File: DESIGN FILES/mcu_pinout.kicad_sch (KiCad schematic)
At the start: 16 parts, among them U1 MIMXRT1064CVL5B

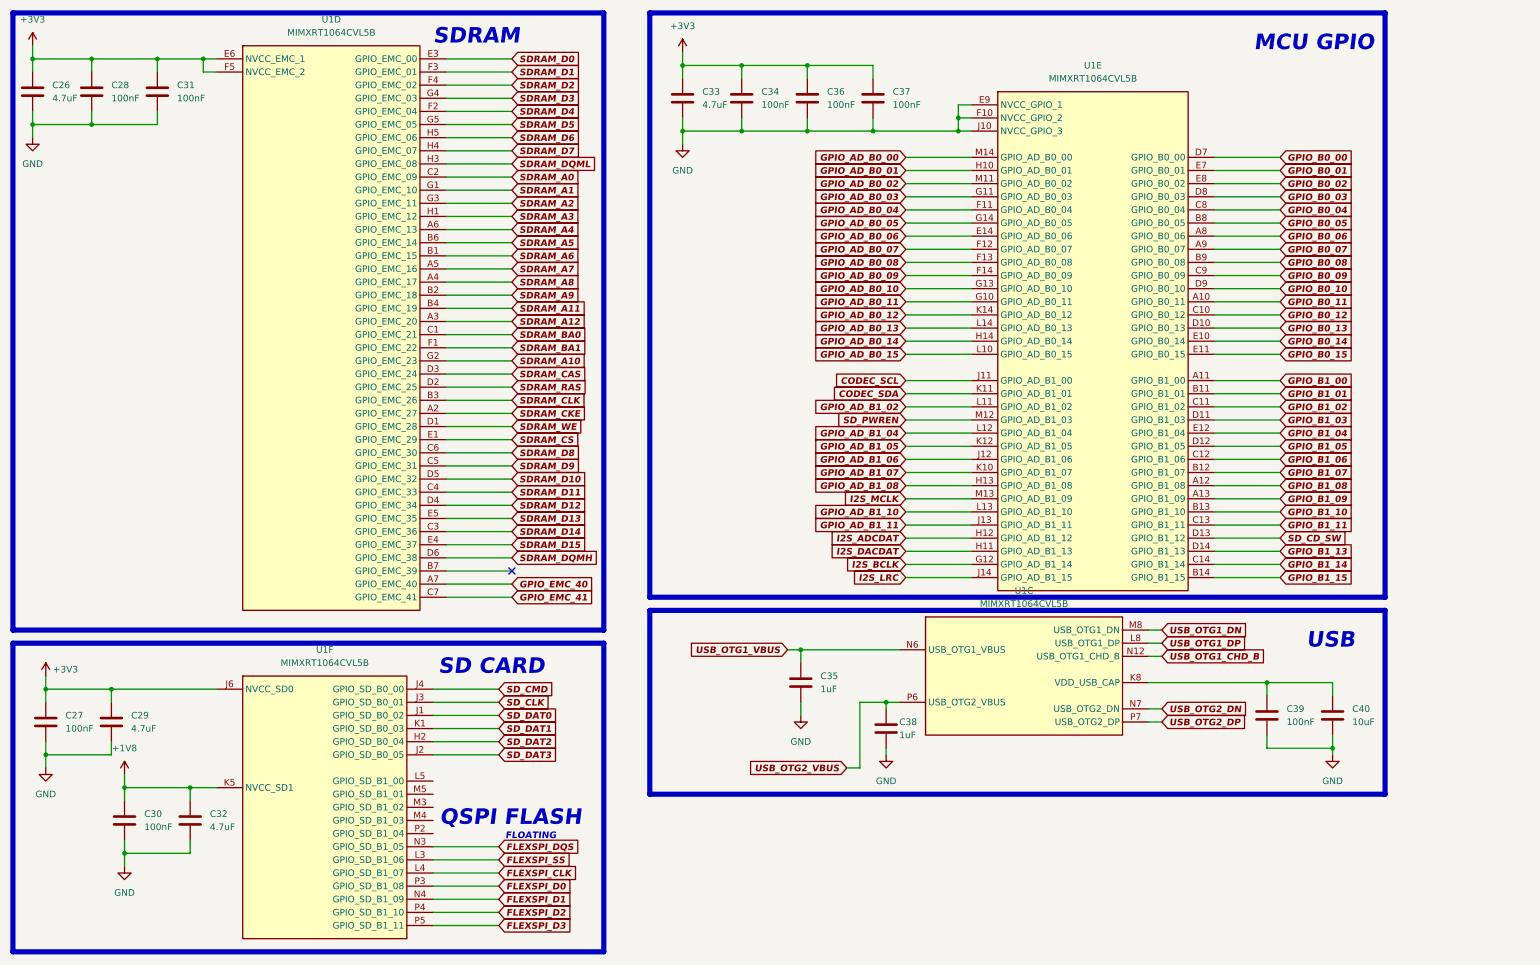
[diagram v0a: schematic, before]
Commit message: work
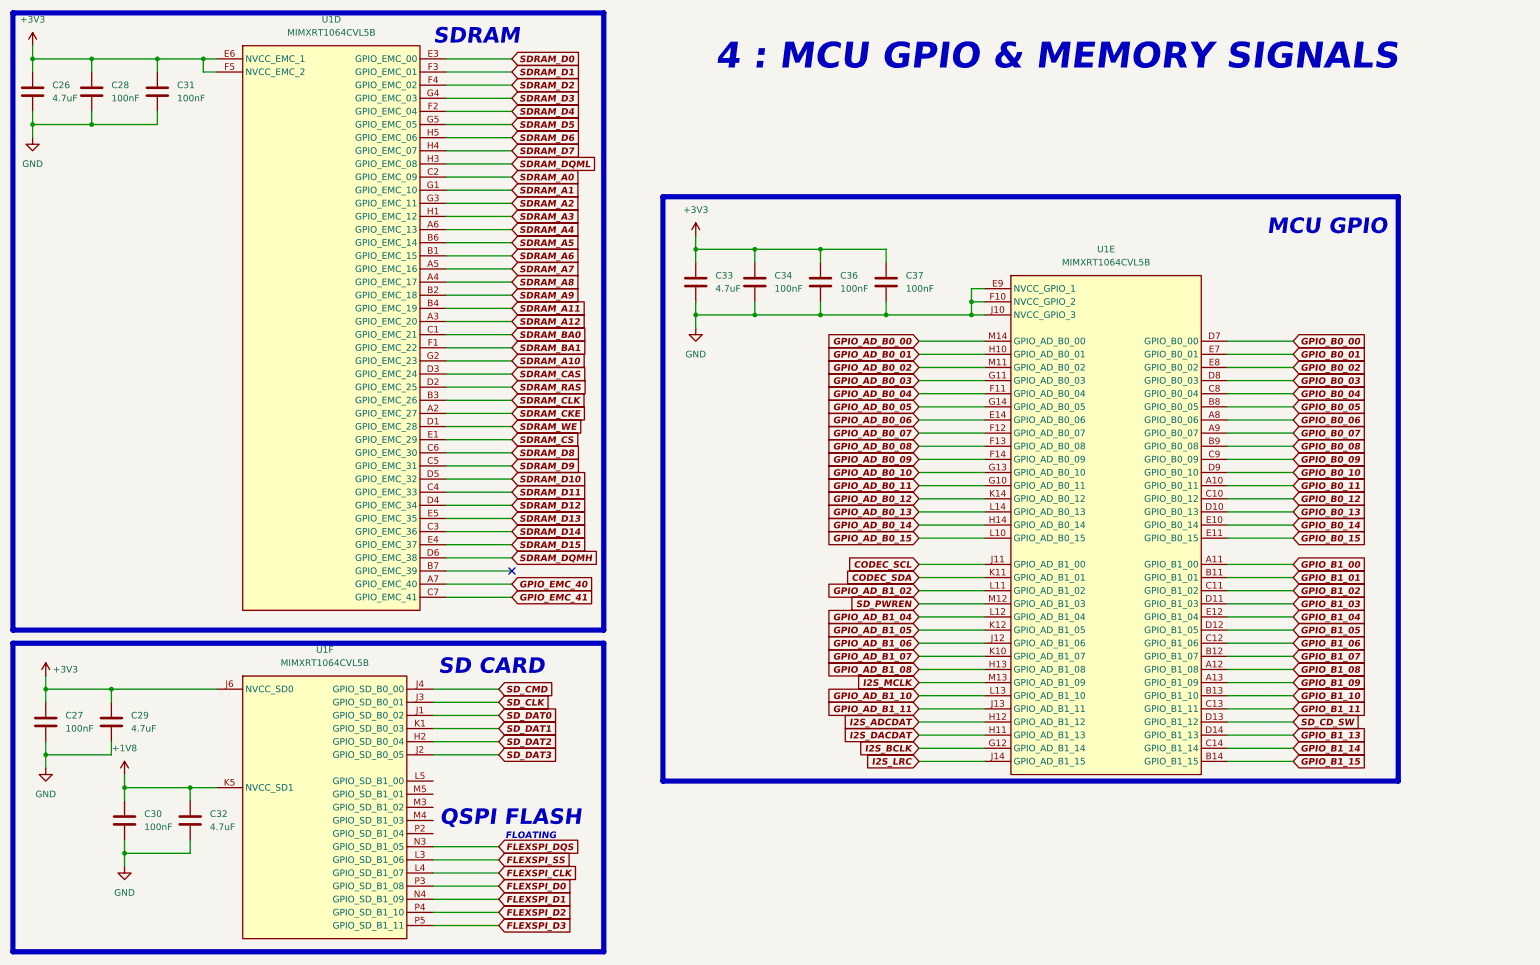
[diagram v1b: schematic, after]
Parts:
- removed C35, C38: 1uF, MIMXRT1064 MCU Module:0402_CL05A105KA5NQNC, symbol MIMXRT1064 MCU Module:CL05A105KA5NQNC
- removed C39: 100nF, MIMXRT1064 MCU Module:0402_CL05B104KB54PNC, symbol MIMXRT1064 MCU Module:CL05B104KB54PNC
- removed C40: 10uF, MIMXRT1064 MCU Module:0603_CL10A106KP8NNNC, symbol MIMXRT1064 MCU Module:CL10A106KP8NNNC
- removed unit 3 of U1
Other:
- note added: "4 : MCU GPIO & MEMORY SIGNALS"
- note removed: "USB"
- company: (none) -> Soundsom
- title: (none) -> MCU GPIO & Memory signals
- moved on the sheet: C33, C34, C36, C37, U1E

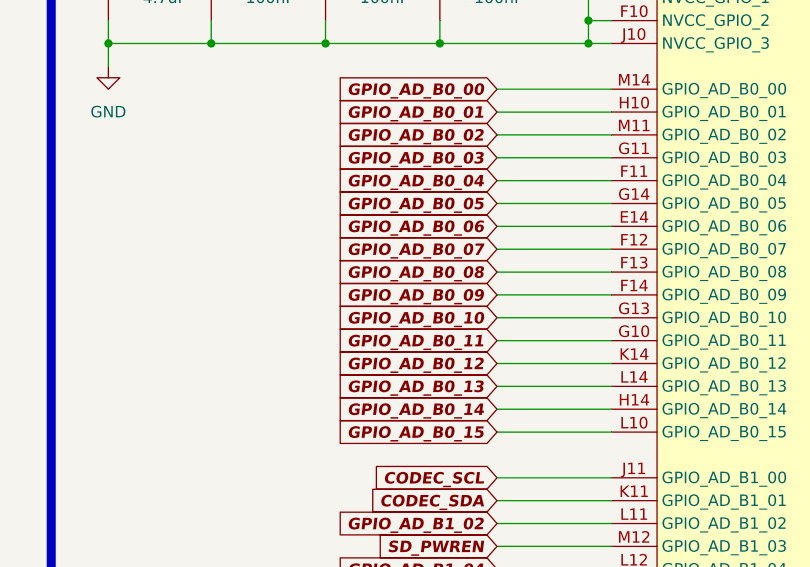
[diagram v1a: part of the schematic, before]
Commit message: schematic edit
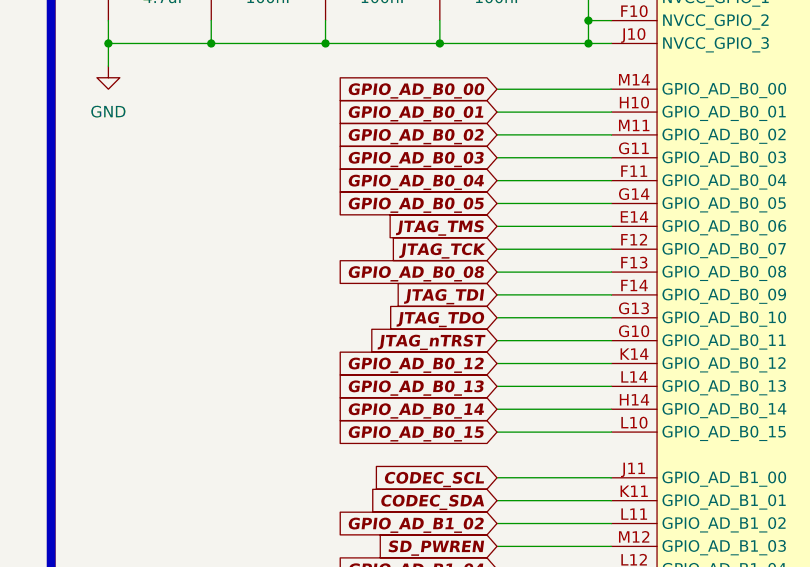
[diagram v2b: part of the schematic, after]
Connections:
- net GPIO_AD_B0_06 renamed JTAG_TMS
- net GPIO_AD_B0_07 renamed JTAG_TCK
- net GPIO_AD_B0_09 renamed JTAG_TDI
- net GPIO_AD_B0_10 renamed JTAG_TDO
- net GPIO_AD_B0_11 renamed JTAG_nTRST
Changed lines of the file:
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@@
     )
   )
-  (global_label "GPIO_AD_B0_06" (shape input) (at 189.23 92.71 180) (fields_autoplaced)
-    (effects (font (size 1.27 1.27) bold italic) (justify right))
-    (property "Intersheet References" "${INTERSHEET_REFS}" (id 0) (at 171.7357 92.583 0)
+  (global_label "JTAG_TMS" (shape input) (at 189.23 92.71 180) (fields_autoplaced)
+    (effects (font (size 1.27 1.27) bold italic) (justify right))
+    (property "Intersheet References" "${INTERSHEET_REFS}" (id 0) (at 177.4809 92.583 0)
       (effects (font (size 1.27 1.27) bold italic) (justify right) hide)
     )
@@
     )
   )
-  (global_label "GPIO_AD_B0_09" (shape input) (at 189.23 100.33 180) (fields_autoplaced)
-    (effects (font (size 1.27 1.27) bold italic) (justify right))
-    (property "Intersheet References" "${INTERSHEET_REFS}" (id 0) (at 171.7357 100.203 0)
+  (global_label "JTAG_TDI" (shape input) (at 189.23 100.33 180) (fields_autoplaced)
+    (effects (font (size 1.27 1.27) bold italic) (justify right))
+    (property "Intersheet References" "${INTERSHEET_REFS}" (id 0) (at 178.2671 100.203 0)
       (effects (font (size 1.27 1.27) bold italic) (justify right) hide)
     )
@@
     )
   )
-  (global_label "GPIO_AD_B0_10" (shape input) (at 189.23 102.87 180) (fields_autoplaced)
-    (effects (font (size 1.27 1.27) bold italic) (justify right))
-    (property "Intersheet References" "${INTERSHEET_REFS}" (id 0) (at 171.7357 102.743 0)
+  (global_label "JTAG_TDO" (shape input) (at 189.23 102.87 180) (fields_autoplaced)
+    (effects (font (size 1.27 1.27) bold italic) (justify right))
+    (property "Intersheet References" "${INTERSHEET_REFS}" (id 0) (at 177.5414 102.743 0)
       (effects (font (size 1.27 1.27) bold italic) (justify right) hide)
     )
@@
     )
   )
-  (global_label "GPIO_AD_B0_11" (shape input) (at 189.23 105.41 180) (fields_autoplaced)
-    (effects (font (size 1.27 1.27) bold italic) (justify right))
-    (property "Intersheet References" "${INTERSHEET_REFS}" (id 0) (at 171.7357 105.283 0)
+  (global_label "JTAG_nTRST" (shape input) (at 189.23 105.41 180) (fields_autoplaced)
+    (effects (font (size 1.27 1.27) bold italic) (justify right))
+    (property "Intersheet References" "${INTERSHEET_REFS}" (id 0) (at 175.5457 105.283 0)
       (effects (font (size 1.27 1.27) bold italic) (justify right) hide)
     )
@@
     )
   )
-  (global_label "GPIO_AD_B0_07" (shape input) (at 189.23 95.25 180) (fields_autoplaced)
-    (effects (font (size 1.27 1.27) bold italic) (justify right))
-    (property "Intersheet References" "${INTERSHEET_REFS}" (id 0) (at 171.7357 95.123 0)
-      (effects (font (size 1.27 1.27) bold italic) (justify right) hide)
-    )
+  (global_label "JTAG_TCK" (shape input) (at 189.23 95.25 180) (fields_autoplaced)
+    (effects (font (size 1.27 1.27) bold italic) (justify right))
+    (property "Intersheet References" "${INTERSHEET_REFS}" (id 0) (at 177.6019 95.123 0)
+      (effects (font (size 1.27 1.27) bold italic) (justify right) hide)
+    )
